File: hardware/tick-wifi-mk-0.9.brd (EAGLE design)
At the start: 96 x 54 mm, 23 parts, among them IC1 MAX7219, IC2 MAX7219

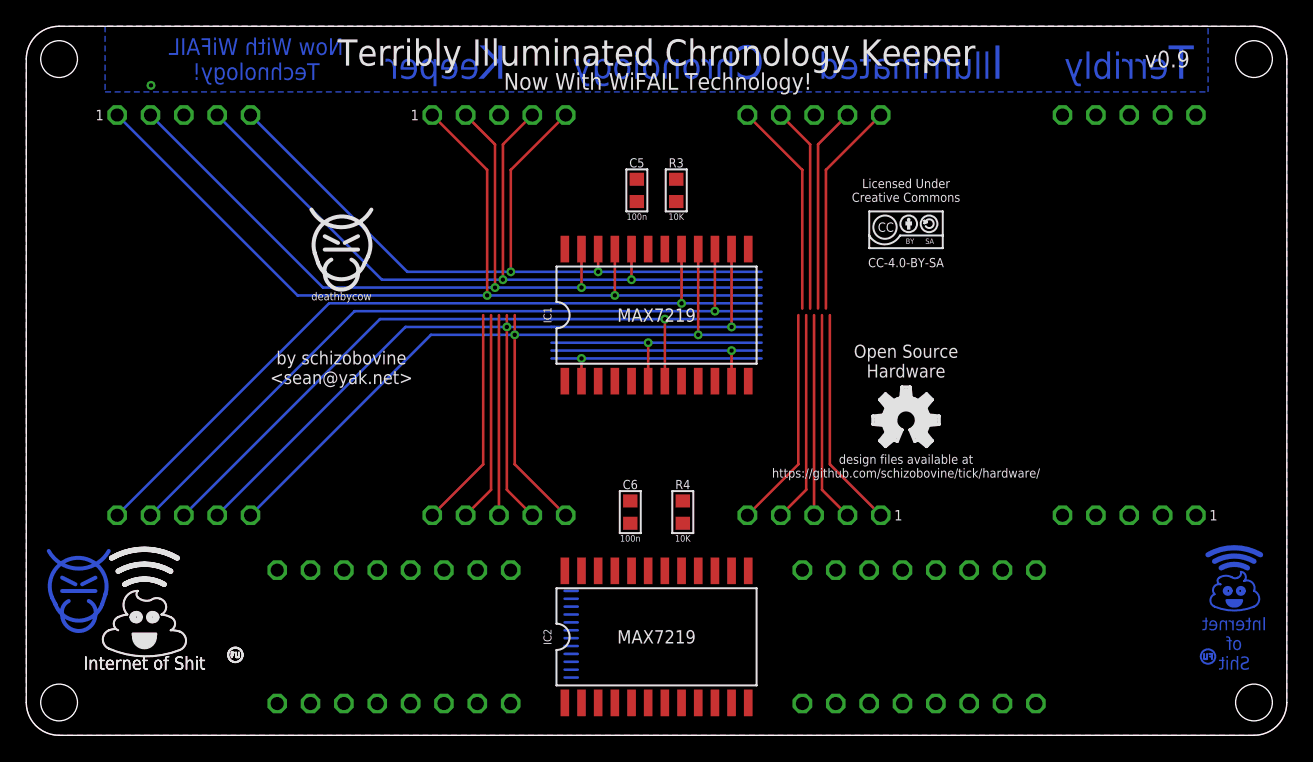
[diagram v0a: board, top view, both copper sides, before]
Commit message: how did this not get commited before?
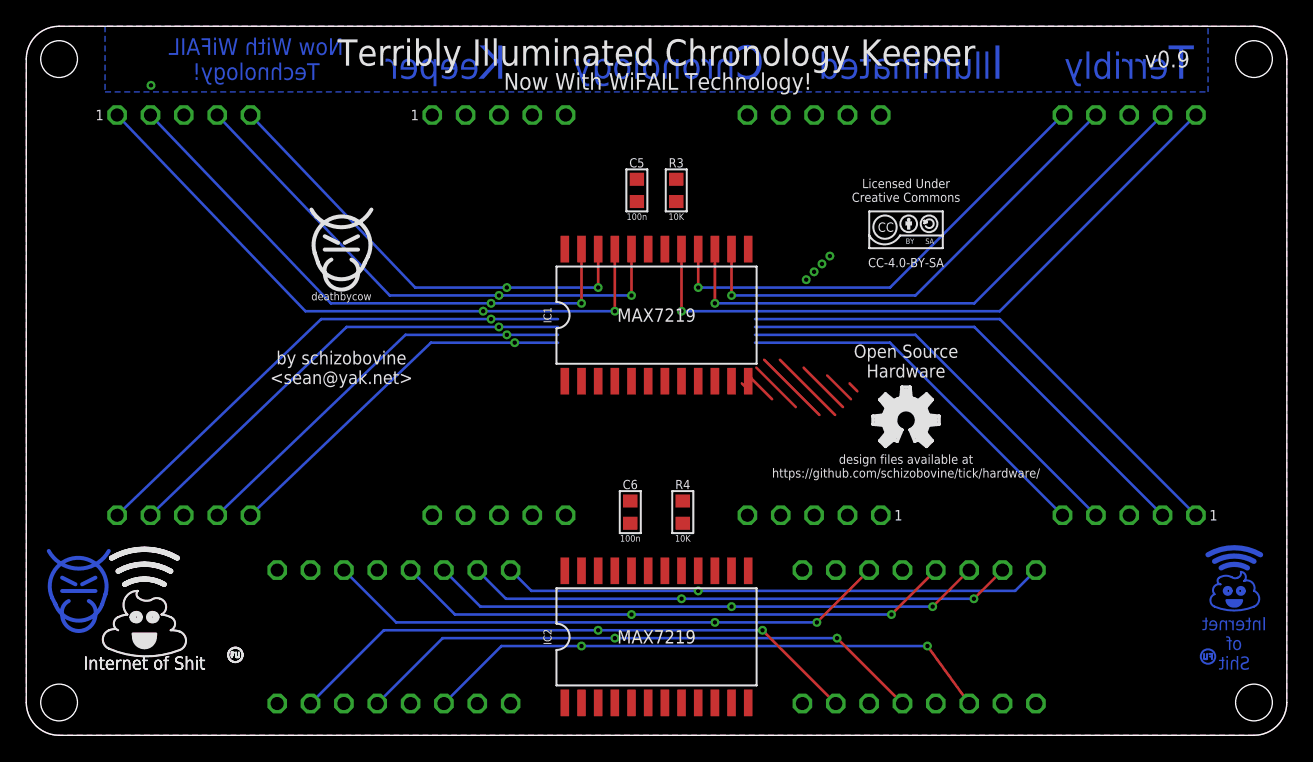
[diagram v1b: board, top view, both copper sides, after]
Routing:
- net DIG_4: track 54.9 -> 0.00 mm, vias 1 -> 0
- net SEG_2P: track 1.00 -> 44.6 mm, vias 0 -> 2
- net SEG_2E: track 1.00 -> 44.1 mm, vias 0 -> 2
- net SEG_2D: track 1.00 -> 44.0 mm, vias 0 -> 2
- net SEG_2F: track 1.00 -> 43.3 mm, vias 0 -> 2
- net SEG_2C: track 1.00 -> 42.8 mm, vias 0 -> 2
- net SEG_2A: track 1.00 -> 42.3 mm, vias 0 -> 2
- net SEG_2G: track 1.00 -> 41.8 mm, vias 0 -> 2
- net SEG_2B: track 1.00 -> 41.3 mm, vias 0 -> 1
- net DIG_3: track 34.2 -> 0.00 mm, vias 1 -> 0
- net DIG_2: track 33.6 -> 0.00 mm, vias 1 -> 0
- net SEG_1B: track 84.5 -> 64.8 mm
- net DIG_1: track 17.7 -> 0.00 mm, vias 1 -> 0
- net SEG_1A: track 85.0 -> 68.4 mm
- net SEG_1P: track 76.1 -> 63.9 mm, vias 2 -> 3
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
